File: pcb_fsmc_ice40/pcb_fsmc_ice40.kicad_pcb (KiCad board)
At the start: 2 copper layers, 76.2 x 32 mm, 40 parts, among them P2 CONN_01X20, P3 CONN_01X20, P4 MICRO-SD, P5 CONN_01X12, P6 CONN_01X12, P7 KNUSB, U1 STM32F40X_LQFP144, X1 CRYSTAL

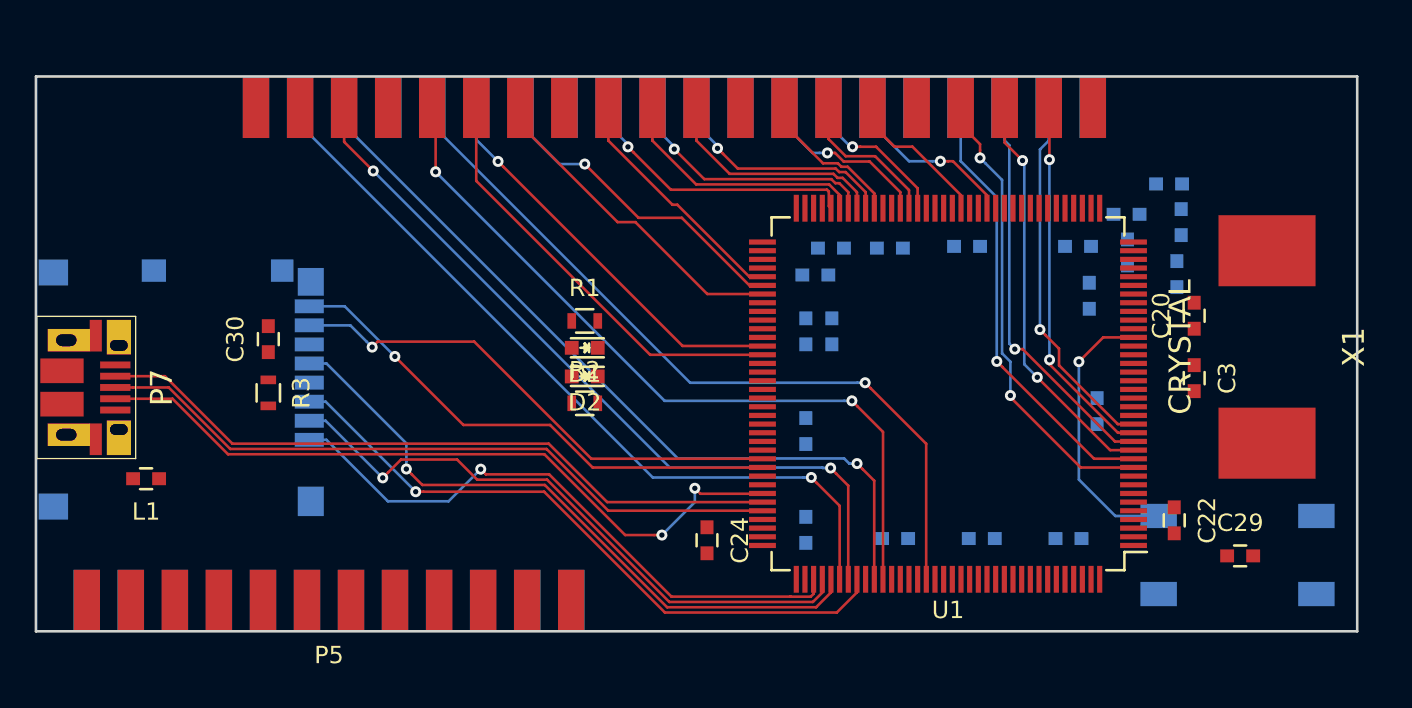
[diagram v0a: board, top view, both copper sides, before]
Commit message: Some more work on PCB, still work left to do.
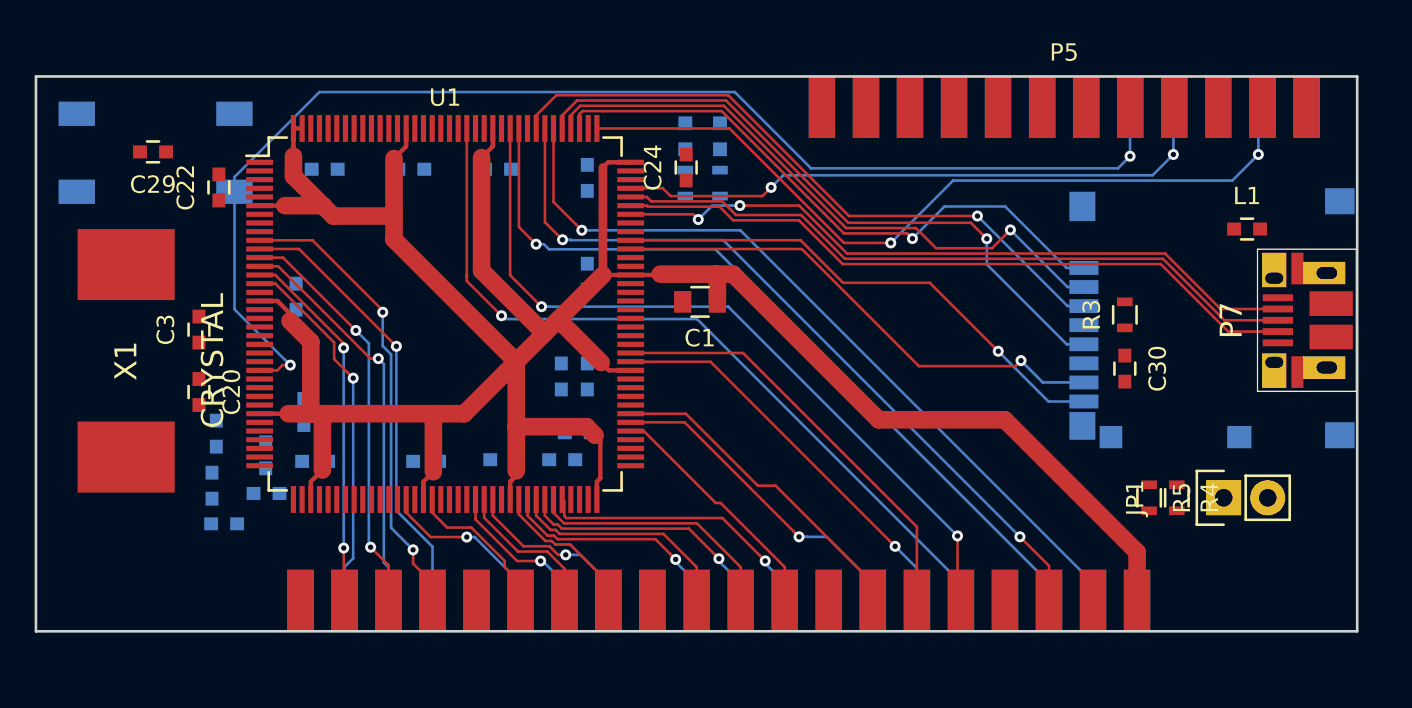
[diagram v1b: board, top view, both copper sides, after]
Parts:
- added C1: 10uF, Capacitors_SMD:C_0805, F.Cu at (138.3, 113.0)
- added JP1: Jumper_NO_Small, Pin_Headers:Pin_Header_Straight_1x02, F.Cu at (168.5, 124.3)
- added R4: 47k, Resistors_SMD:R_0603, F.Cu at (165.8, 124.3)
- added R5: 47k, Resistors_SMD:R_0603, F.Cu at (164.2, 124.3)
- D1, D2, R1, R2: moved to B.Cu
- moved P7 72.8 mm to (174.5, 114.1), turned to 90 degrees
- moved C29 66.9 mm to (106.8, 104.3), turned to 180 degrees
- moved B1 66.6 mm to (106.9, 104.4), turned to 270 degrees
- moved X1 65.8 mm to (105.2, 116.4), turned to 90 degrees
- moved L1 65.1 mm to (169.8, 108.8), turned to 0 degrees
- moved P4 59.1 mm to (167.6, 113.9), turned to 90 degrees
- moved C22 58.3 mm to (110.6, 106.4), turned to 90 degrees
- moved C28 57.9 mm to (110.2, 123.6), turned to 270 degrees
- moved L2 57.9 mm to (110.8, 125.8), turned to 0 degrees
- moved C20 57.6 mm to (109.4, 118.2), turned to 270 degrees
- moved C3 57.5 mm to (109.4, 114.6), turned to 90 degrees
- moved C27 56.2 mm to (110.4, 120.6), turned to 90 degrees
- moved C26 52.1 mm to (113.3, 124.0), turned to 180 degrees
- moved C25 51.1 mm to (113.2, 121.8), turned to 90 degrees
- moved P5 51.0 mm to (159.3, 101.8), turned to 180 degrees
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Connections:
- P5 pad 1: +3.3V -> Net-(P5-Pad1)
- P5 pad 2: /swclk -> Net-(P5-Pad2)
- P5 pad 3: GND -> Net-(P5-Pad3)
- P5 pad 4: /swdio -> Net-(P5-Pad4)
- P5 pad 5: /nrst -> Net-(P5-Pad5)
- P5 pad 6: /swo -> Net-(P5-Pad6)
- P6 pad 1: Net-(P6-Pad1) -> +3.3V
- P6 pad 2: Net-(P6-Pad2) -> /swclk
- P6 pad 3: Net-(P6-Pad3) -> GND
- P6 pad 4: Net-(P6-Pad4) -> /swdio
- P6 pad 5: Net-(P6-Pad5) -> /nrst
- U1 pad 138: GND -> /boot0
- U1 pad 48: /pb2 -> /boot1
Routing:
- net +3.3V: track 0.00 -> 157.9 mm
- net /nrst: track 15.9 -> 72.6 mm, vias 1 -> 2
- net /swclk: track 0.00 -> 45.5 mm, vias 0 -> 2
- net /swdio: track 0.00 -> 35.1 mm, vias 0 -> 2
- net /usb_id: track 42.4 -> 40.3 mm
- net /sram2_ce: track 44.8 -> 45.6 mm
- added copper zone on B.Cu, net GND
- added copper zone on F.Cu, net GND
